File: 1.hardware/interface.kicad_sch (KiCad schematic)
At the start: 36 parts, among them J1 Conn_01x02, J12 Conn_01x02, J13 Conn_01x02, J14 Conn_01x03, J16 Can_conn, J7 uart_comm, J8 USB_C, SW1 Esp32_Btn, U11 SN65HVD230, U5 ESP32-C3-WROOM-02

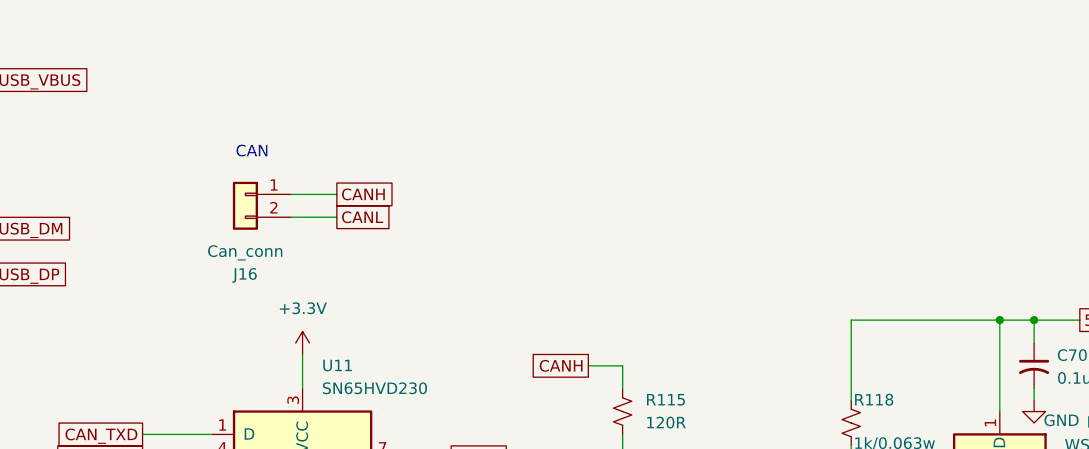
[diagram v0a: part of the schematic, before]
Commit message: 중간 수정
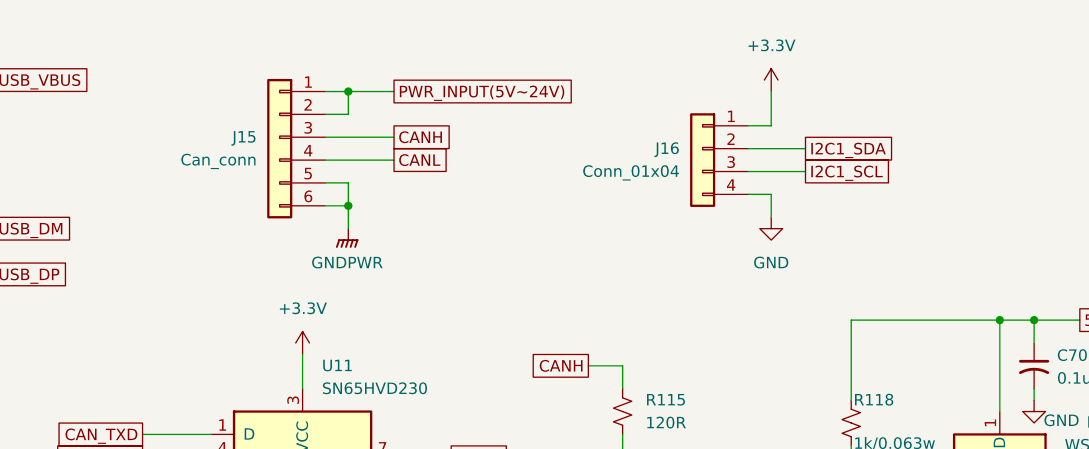
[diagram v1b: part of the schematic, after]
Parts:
- removed J16: Can_conn, symbol Connector_Generic:Conn_01x02
- added J15: Can_conn, symbol Connector_Generic:Conn_01x06
- added J16: Conn_01x04, symbol Connector_Generic:Conn_01x04
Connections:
- net +3.3V: now also J16.1 (Pin_1)
- net CANH: now also J15.3 (Pin_3)
- net CANL: now also J15.4 (Pin_4)
- net GND: now also J16.4 (Pin_4)
- new net GNDPWR: J15.5 (Pin_5), J15.6 (Pin_6)
- new net I2C1_SCL: J16.3 (Pin_3)
- new net I2C1_SDA: J16.2 (Pin_2)
- new net PWR_INPUT(5V~24V): J15.1 (Pin_1), J15.2 (Pin_2)
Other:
- note removed: "CAN"
